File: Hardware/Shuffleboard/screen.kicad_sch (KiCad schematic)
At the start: 1 part, among them U7 Adafruit ST7735R

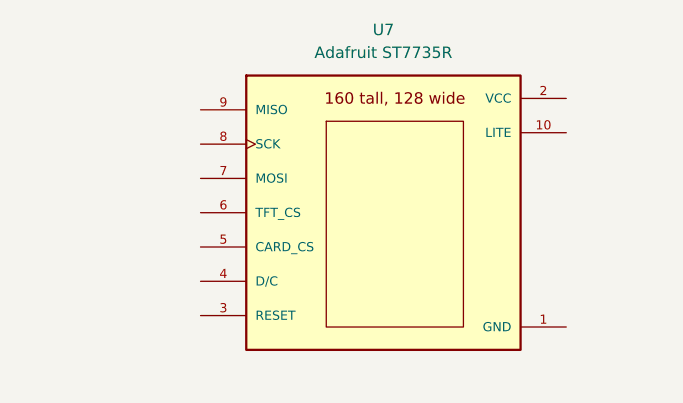
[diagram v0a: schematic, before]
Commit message: Finished Screen
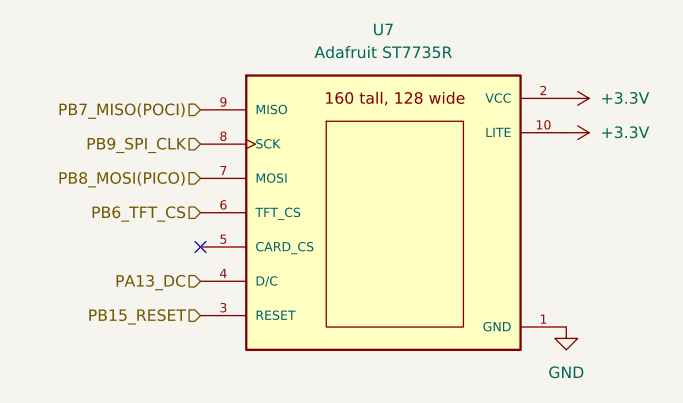
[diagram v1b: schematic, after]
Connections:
- net GND: now reaches U7.1 (GND)
- net +3.3V: now reaches U7.10 (LITE)
- net +3.3V: now also U7.2 (VCC)
- net PB15_RESET: now reaches U7.3 (RESET)
- net PA13_DC: now reaches U7.4 (D/C)
- net PB6_TFT_CS: now reaches U7.6 (TFT_CS)
- net PB8_MOSI(PICO): now reaches U7.7 (MOSI)
- net PB9_SPI_CLK: now reaches U7.8 (SCK)
- net PB7_MISO(POCI): now reaches U7.9 (MISO)
- no-connect marks 0 -> 1
